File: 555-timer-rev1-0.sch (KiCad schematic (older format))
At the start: 19 parts, among them J1 Conn_01x02_Male, SW1 SW_Push, SW2 SW_Push, U1 SA555D

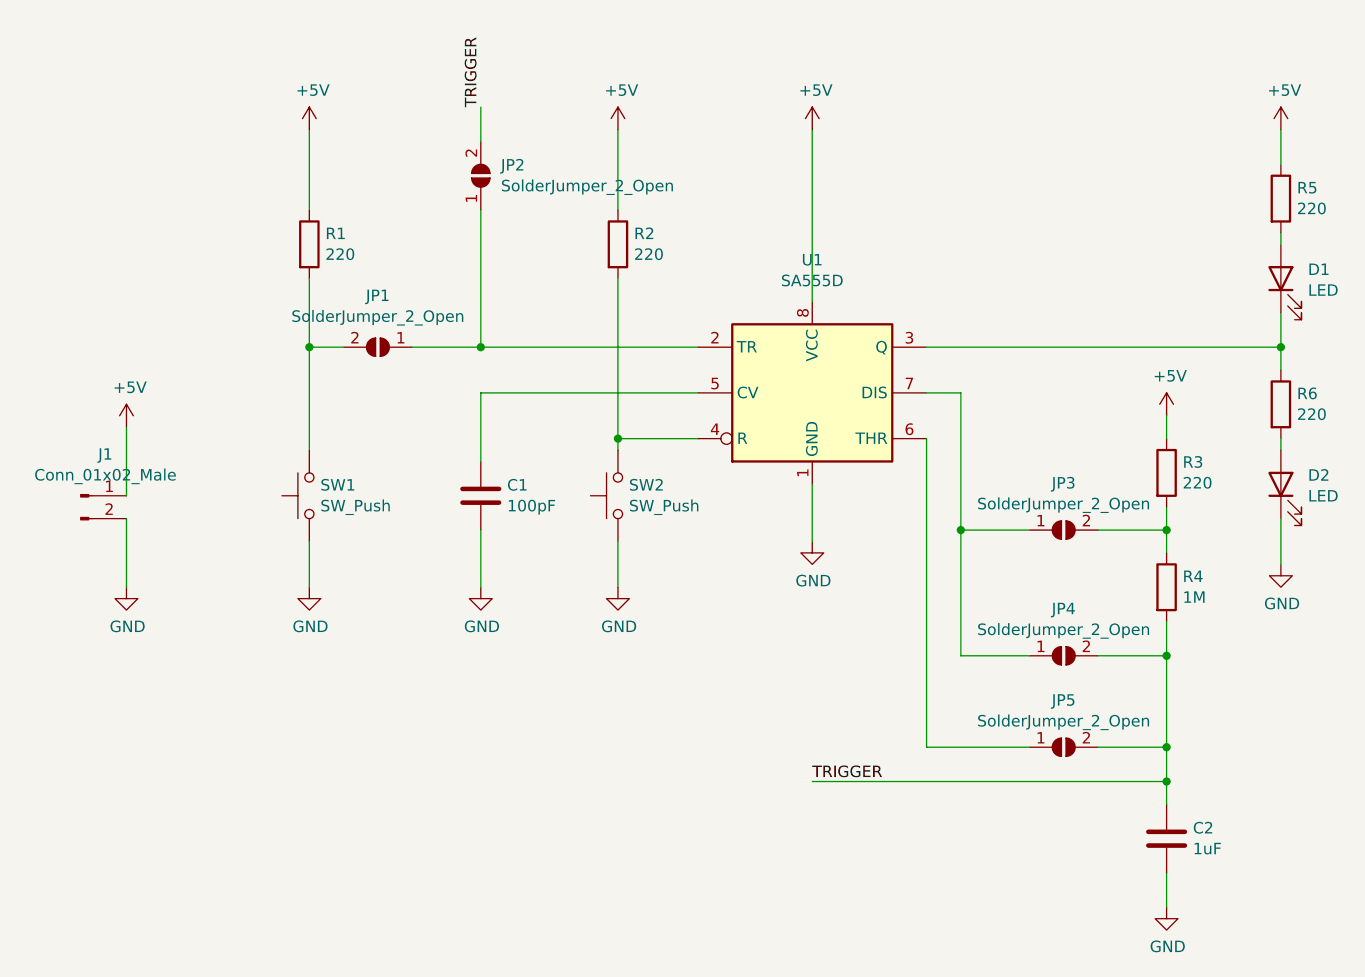
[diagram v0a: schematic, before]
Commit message: Finish PCB layout.
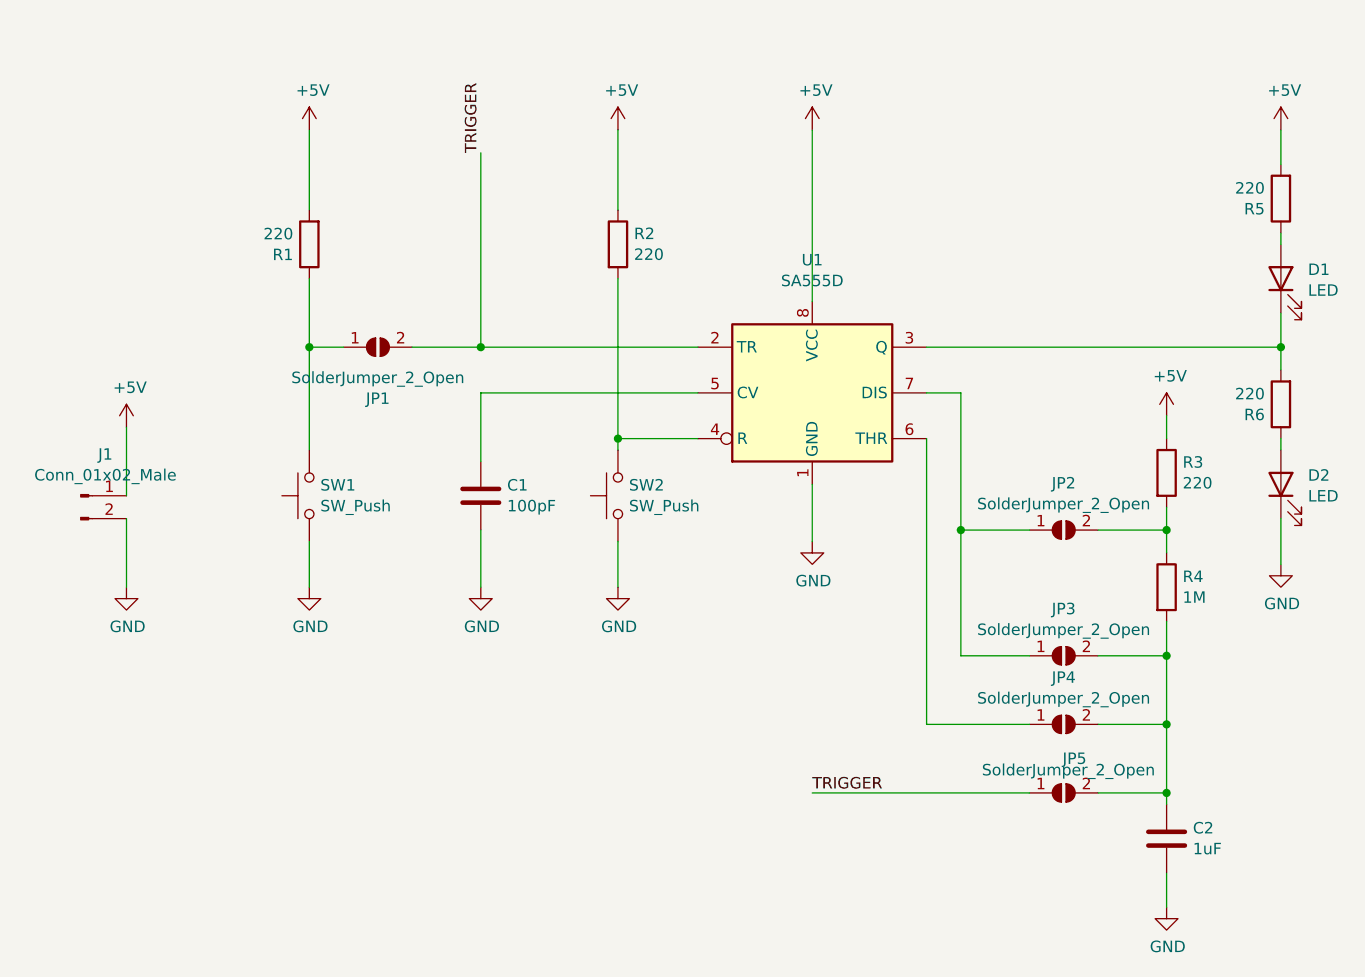
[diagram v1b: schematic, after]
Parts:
- renumbered JP3 to JP2, JP4 to JP3, JP5 to JP4, JP2 to JP5
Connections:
- net +5V: now also R1.2, R5.2; no longer R1.1, R5.1
- net TRIGGER: now also JP1.2 (B), JP5.1 (A), U1.2 (TR); no longer C2.1, JP3.2 (B), JP4.2 (B), JP5.2 (B), R4.2
- net at D1.1 (K), U1.3 (Q): now also R6.2; no longer R6.1
- net at D1.2 (A): now also R5.1; no longer R5.2
- net at D2.2 (A): now also R6.1; no longer R6.2
- new net: C2.1, JP3.2 (B), JP4.2 (B), JP5.2 (B), R4.2
- new net: JP1.1 (A), R1.1, SW1.2
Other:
- moved on the sheet: JP4, JP5
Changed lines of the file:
@@
 F 3 "~" H 8050 3150 50  0001 C CNN
 	1    8050 3150
-	1    0    0    -1
+	-1   0    0    1
 $EndComp
 $Comp
@@
 F 3 "~" H 8050 4050 50  0001 C CNN
 	1    8050 4050
-	1    0    0    -1
+	-1   0    0    1
 $EndComp
 $Comp
@@
 Wire Wire Line
 	7550 4500 7550 4600
-Wire Wire Line
-	7550 5000 7550 5150
 Connection ~ 7550 4600
 Wire Wire Line
 	7550 4600 7550 4700
-Connection ~ 7550 5550
+Connection ~ 7550 5450
 $Comp
 L power:GND #PWR011
@@
 	6650 4000 6650 4600
 Wire Wire Line
-	6500 4200 6500 5550
-Wire Wire Line
 	4550 4000 4550 4300
 Wire Wire Line
@@
 Wire Wire Line
 	8050 3800 8050 3900
-Text Label 6000 5700 0    50   ~ 0
+Text Label 6000 5750 0    50   ~ 0
 TRIGGER
 $Comp
@@
 F 3 "~" H 3800 3350 50  0001 C CNN
 	1    3800 3350
-	1    0    0    -1
+	-1   0    0    1
 $EndComp
 $Comp
@@
 F 3 "~" H 4100 3800 50  0001 C CNN
 	1    4100 3800
-	-1   0    0    1
+	1    0    0    -1
 $EndComp
 Wire Wire Line
@@
 Wire Wire Line
 	5150 4200 5150 4250
-Wire Wire Line
-	7550 5550 7550 5700
-Connection ~ 7550 5700
 Wire Wire Line
 	6650 4600 6650 5150
 Connection ~ 6650 4600
 Connection ~ 7550 5150
-Wire Wire Line
-	7550 5150 7550 5550
-$Comp
-L Jumper:SolderJumper_2_Open JP3
+$Comp
+L Jumper:SolderJumper_2_Open JP2
 U 1 1 5F2FC22B
 P 7100 4600
-F 0 "JP3" H 7100 4805 50  0000 C CNN
+F 0 "JP2" H 7100 4805 50  0000 C CNN
 F 1 "SolderJumper_2_Open" H 7100 4714 50  0000 C CNN
 F 2 "Jumper:SolderJumper-2_P1.3mm_Open_TrianglePad1.0x1.5mm" H 7100 4600 50  0001 C CNN
@@
 	7250 4600 7550 4600
 $Comp
-L Jumper:SolderJumper_2_Open JP4
+L Jumper:SolderJumper_2_Open JP3
 U 1 1 5F2FCB39
 P 7100 5150
-F 0 "JP4" H 7100 5355 50  0000 C CNN
+F 0 "JP3" H 7100 5355 50  0000 C CNN
 F 1 "SolderJumper_2_Open" H 7100 5264 50  0000 C CNN
 F 2 "Jumper:SolderJumper-2_P1.3mm_Open_TrianglePad1.0x1.5mm" H 7100 5150 50  0001 C CNN
@@
 	6500 3800 8050 3800
 Wire Wire Line
-	6000 5700 7550 5700
-Wire Wire Line
-	6500 5550 6950 5550
+	6000 5750 6950 5750
+Wire Wire Line
+	6500 5450 6950 5450
 Wire Wire Line
 	6650 5150 6950 5150
@@
 	6650 4600 6950 4600
 Wire Wire Line
-	7550 5700 7550 5800
+	7550 5750 7550 5800
 Wire Wire Line
 	7550 6100 7550 6250
 $Comp
-L Jumper:SolderJumper_2_Open JP5
+L Jumper:SolderJumper_2_Open JP4
 U 1 1 5F3182F6
-P 7100 5550
-F 0 "JP5" H 7100 5755 50  0000 C CNN
-F 1 "SolderJumper_2_Open" H 7100 5664 50  0000 C CNN
-F 2 "Jumper:SolderJumper-2_P1.3mm_Open_TrianglePad1.0x1.5mm" H 7100 5550 50  0001 C CNN
-F 3 "~" H 7100 5550 50  0001 C CNN
-	1    7100 5550
-	1    0    0    -1
-$EndComp
-Wire Wire Line
-	7250 5550 7550 5550
+P 7100 5450
+F 0 "JP4" H 7100 5655 50  0000 C CNN
+F 1 "SolderJumper_2_Open" H 7100 5564 50  0000 C CNN
+F 2 "Jumper:SolderJumper-2_P1.3mm_Open_TrianglePad1.0x1.5mm" H 7100 5450 50  0001 C CNN
+F 3 "~" H 7100 5450 50  0001 C CNN
+	1    7100 5450
+	1    0    0    -1
+$EndComp
+Wire Wire Line
+	7250 5450 7550 5450
 $Comp
 L Connector:Conn_01x02_Male J1
@@
 Wire Wire Line
 	4250 3800 4550 3800
-Text Label 4550 2750 1    50   ~ 0
+Text Label 4550 2950 1    50   ~ 0
 TRIGGER
-Wire Wire Line
-	4550 3800 4550 3200
-$Comp
-L Jumper:SolderJumper_2_Open JP2
+$Comp
+L Jumper:SolderJumper_2_Open JP5
 U 1 1 5F2E91E4
-P 4550 3050
-F 0 "JP2" V 4596 2962 50  0000 R CNN
-F 1 "SolderJumper_2_Open" V 4505 2962 50  0000 R CNN
-F 2 "Jumper:SolderJumper-2_P1.3mm_Open_TrianglePad1.0x1.5mm" H 4550 3050 50  0001 C CNN
-F 3 "~" H 4550 3050 50  0001 C CNN
-	1    4550 3050
-	0    -1   -1   0
-$EndComp
-Wire Wire Line
-	4550 2900 4550 2750
+P 7100 5750
+F 0 "JP5" H 7200 5900 50  0000 R CNN
+F 1 "SolderJumper_2_Open" H 7500 5850 50  0000 R CNN
+F 2 "Jumper:SolderJumper-2_P1.3mm_Open_TrianglePad1.0x1.5mm" H 7100 5750 50  0001 C CNN
+F 3 "~" H 7100 5750 50  0001 C CNN
+	1    7100 5750
+	1    0    0    -1
+$EndComp
 $Comp
 L Switch:SW_Push SW1
@@
 	4550 3800 5500 3800
 Connection ~ 4550 3800
+Wire Wire Line
+	7250 5750 7550 5750
+Wire Wire Line
+	4550 2950 4550 3800
+Wire Wire Line
+	6500 4200 6500 5450
+Wire Wire Line
+	7550 5150 7550 5450
+Wire Wire Line
+	7550 5450 7550 5750
+Wire Wire Line
+	7550 5000 7550 5150
+Connection ~ 7550 5750
 $EndSCHEMATC
